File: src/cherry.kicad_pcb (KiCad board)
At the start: 2 copper layers, 50 x 35 mm, 4 parts

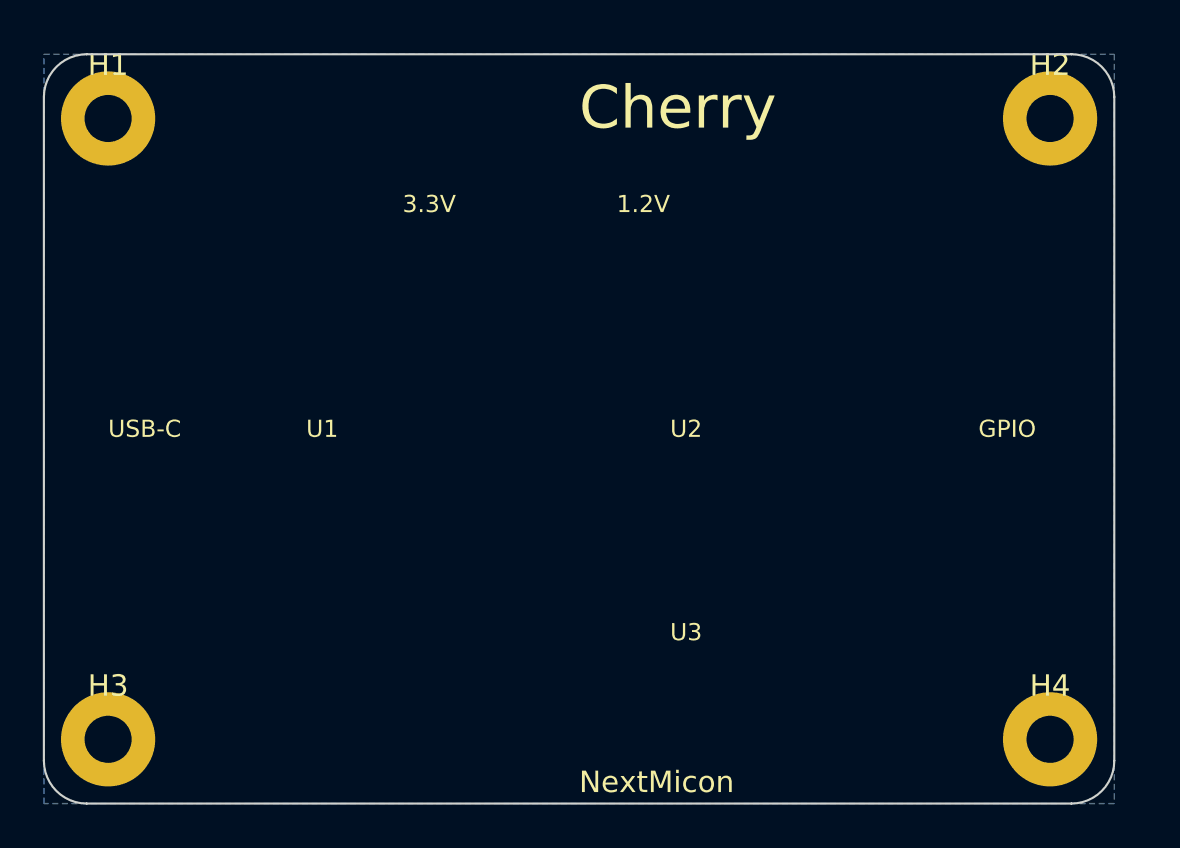
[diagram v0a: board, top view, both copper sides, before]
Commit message: chore
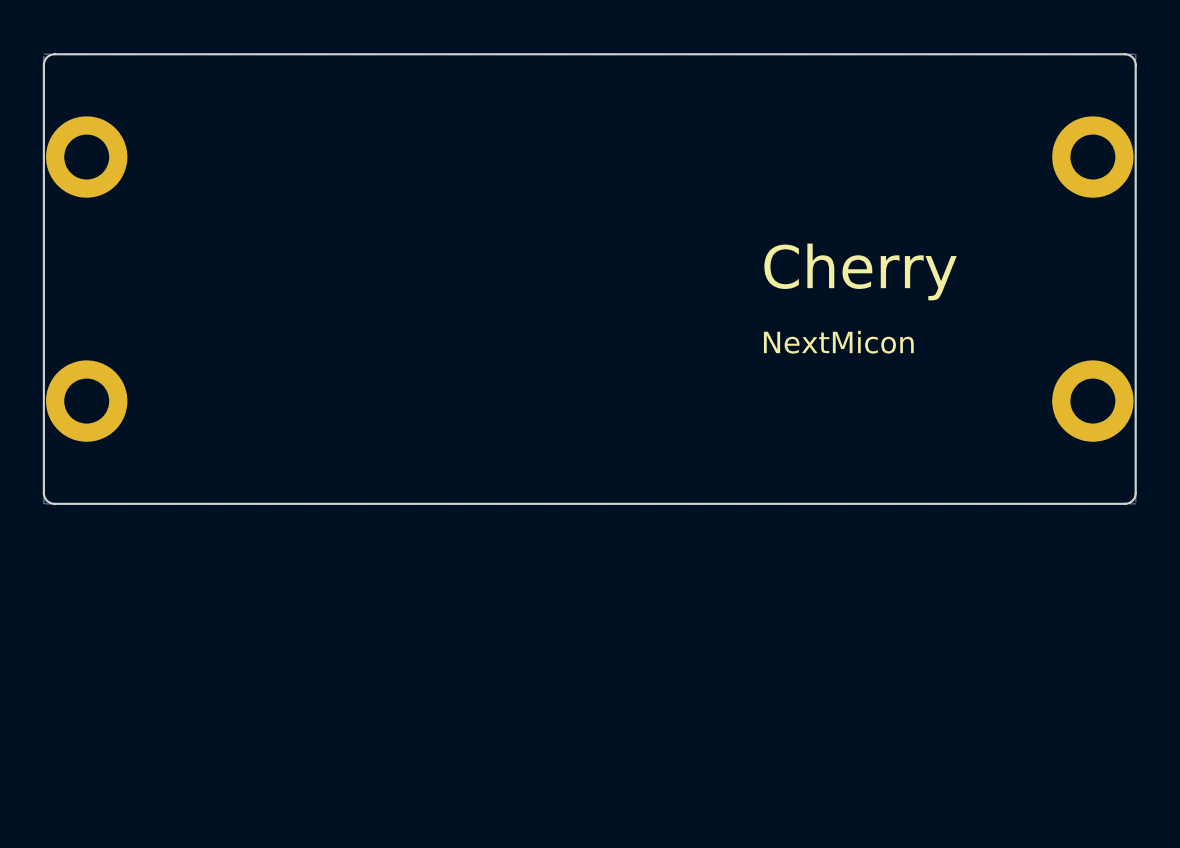
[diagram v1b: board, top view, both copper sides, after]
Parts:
- H1, H2, H3, H4: footprint MountingHole:MountingHole_2.2mm_M2 -> Cherry:MountingHole_2.1mm_M2
- moved H4 15.9 mm to (149.0, 96.2)
- moved H3 15.8 mm to (102.0, 96.2)
- moved H2 2.69 mm to (149.0, 84.8)
- moved H1 2.06 mm to (102.0, 84.8)
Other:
- board size 50 x 35 mm -> 51 x 21 mm
- net class Default removed
- net class Power removed
- net class USB removed
- board text removed: "1.2V"
- board text removed: "3.3V"
- board text removed: "COMPONENT PLACEMENT: J1(USB-C): left edge U1(FT2232H): center-left U2(iCE40): center-right U3(Flash): below U2 U4(3.3V): top center-left U5(1.2V): top center-right J2(GPIO): right edge"
- board text removed: "GPIO"
- board text removed: "U1"
- board text removed: "U2"
- board text removed: "U3"
- board text removed: "USB-C"
